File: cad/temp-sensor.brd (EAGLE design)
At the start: 72.1 x 40.6 mm, 61 parts, among them Q1 300S14-U, Q2 320S14-U, Q3 320S14-U, U1 SE555D, U2 SE555D, U4 MCP6001UT-I/OT, U6 MCP6001UT-I/OT, U7 MCP6001UT-I/OT, U8 NCV4264-2CST50T3G, U9 ATMEGA328P_TQFP, Y1 16MHz

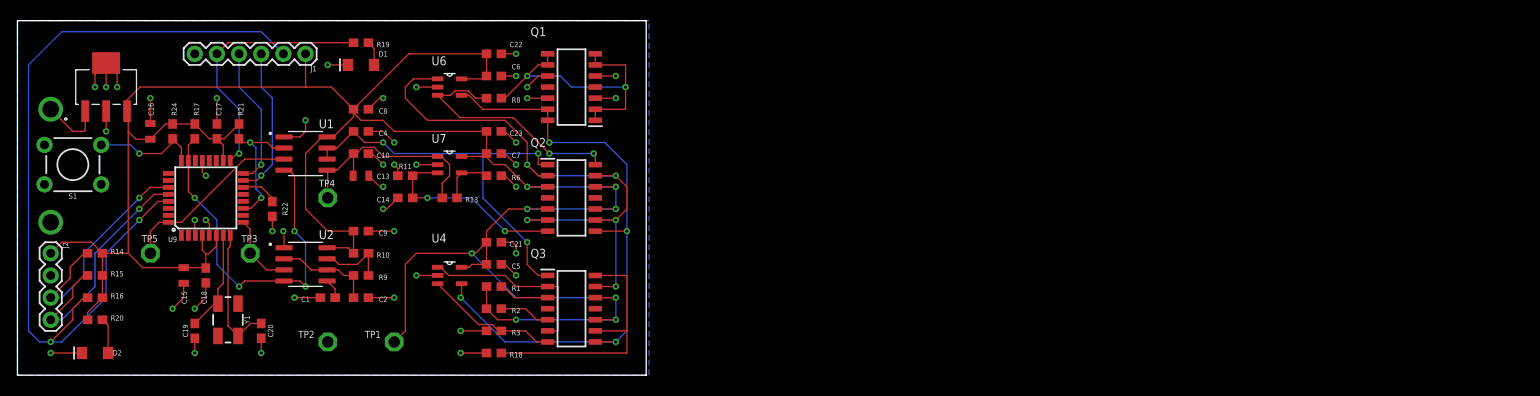
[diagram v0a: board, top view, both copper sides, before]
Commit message: Add files via upload
Implemented plate extension for temperature reading
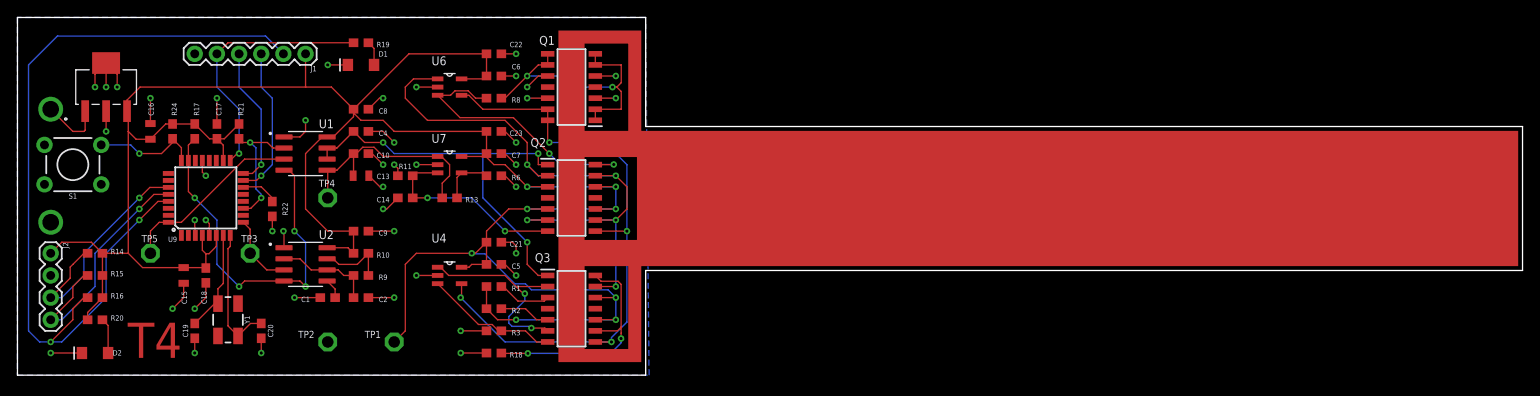
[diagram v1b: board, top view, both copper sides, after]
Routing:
- net PTAT_IN+: track 28.2 -> 31.7 mm
- net START_C: track 30.5 -> 27.5 mm, vias 0 -> 2
- net CTAT_BASE: track 21.1 -> 23.8 mm, vias 0 -> 2
- net 3_NPN_DIODE: track 34.5 -> 32.9 mm
- net TEMP_VBE: track 72.7 -> 71.9 mm
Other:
- board size 72.1 x 40.6 mm -> 172.5 x 41 mm
- board text added: "T4"
